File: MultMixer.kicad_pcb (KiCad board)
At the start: 2 copper layers, 50 x 150 mm, 51 parts, among them J1 Mult IN, J10 In 3, J11 In 4, J12 In 5, J13 Mixer Out, J2 Conn_02x05_Odd_Even, J3 Out 1, J4 Out 2, J5 Out 4, J6 Out 3, J7 Out 5, J8 In 1, J9 In 2, SW1 on/off, SW2 on/off, SW3 on/off, SW4 on/off, SW5 on/off, U1 TL074, U2 TL074

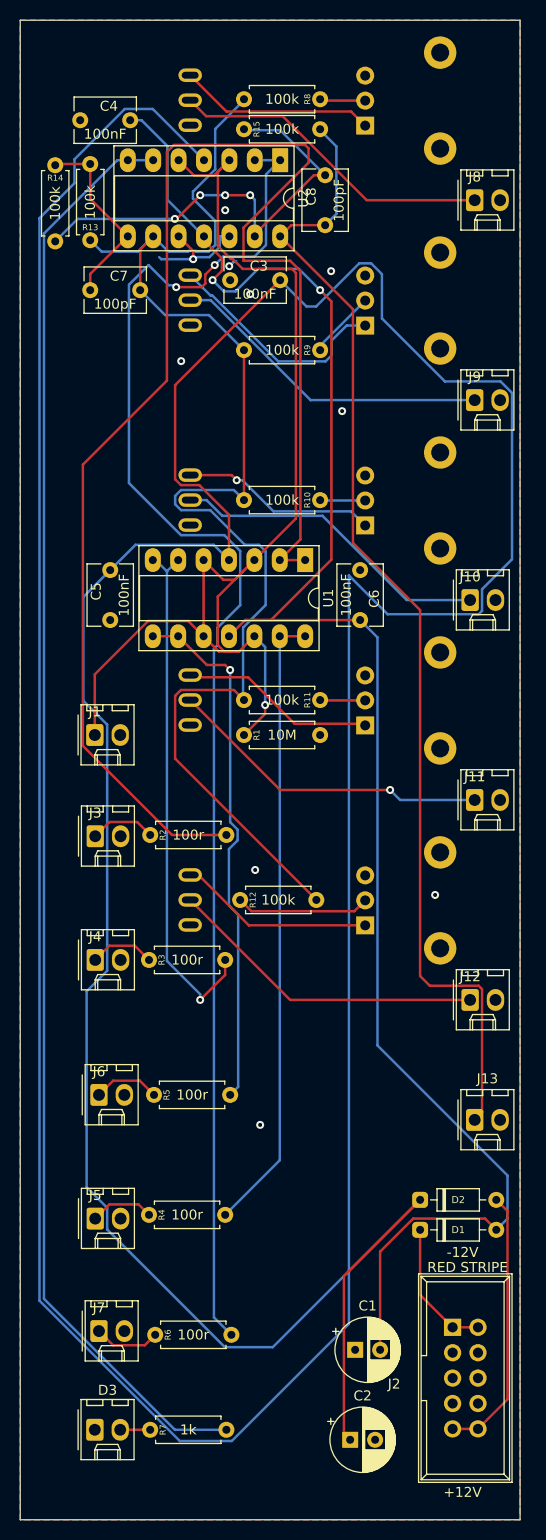
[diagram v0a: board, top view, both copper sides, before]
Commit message: silksmooth
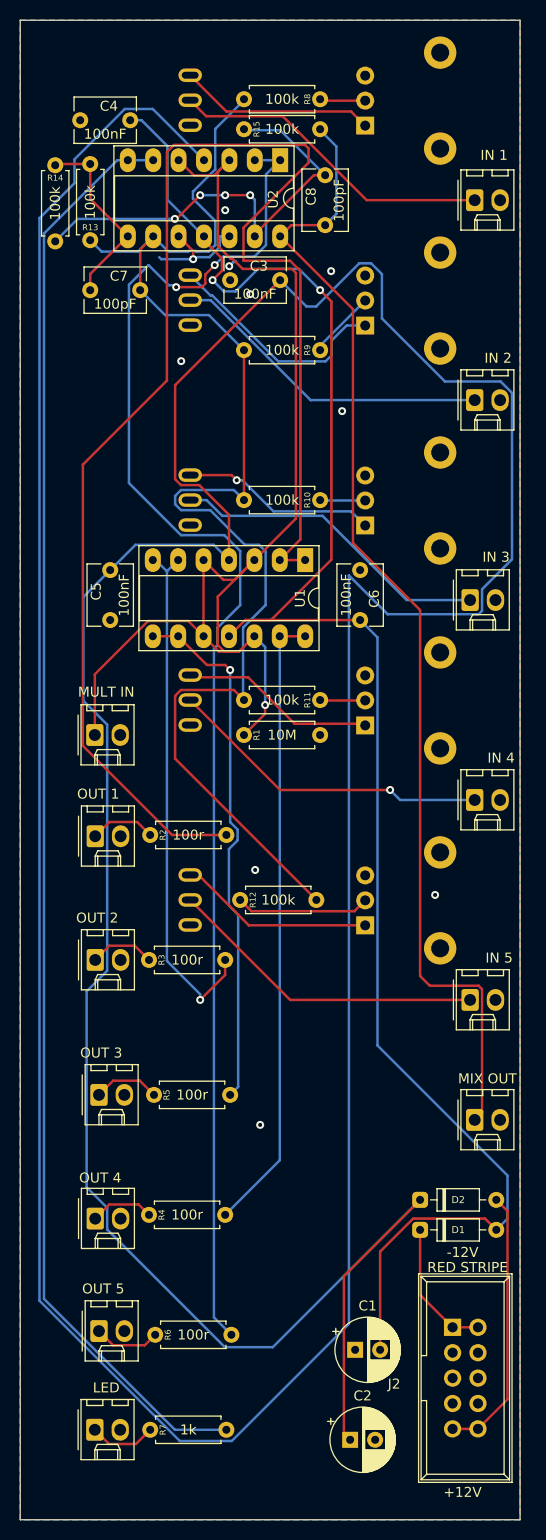
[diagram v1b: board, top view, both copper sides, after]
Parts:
- IN 1: renamed from J8
- IN 2: renamed from J9
- IN 3: renamed from J10
- IN 4: renamed from J11
- IN 5: renamed from J12
- MIX OUT: renamed from J13
- MULT IN: renamed from J1
- OUT 1: renamed from J3
- OUT 2: renamed from J4
- OUT 3: renamed from J6
- OUT 4: renamed from J5
- OUT 5: renamed from J7
- renumbered D3 to LED
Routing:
- net Net-(D3-Pad2): track 3.00 -> 6.72 mm
